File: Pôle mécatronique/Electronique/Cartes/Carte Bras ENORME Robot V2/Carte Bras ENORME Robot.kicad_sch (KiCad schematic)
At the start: 25 parts, among them Q1 BC557, U1 MCP2551-I-P, U2 IRFZ44NPBF

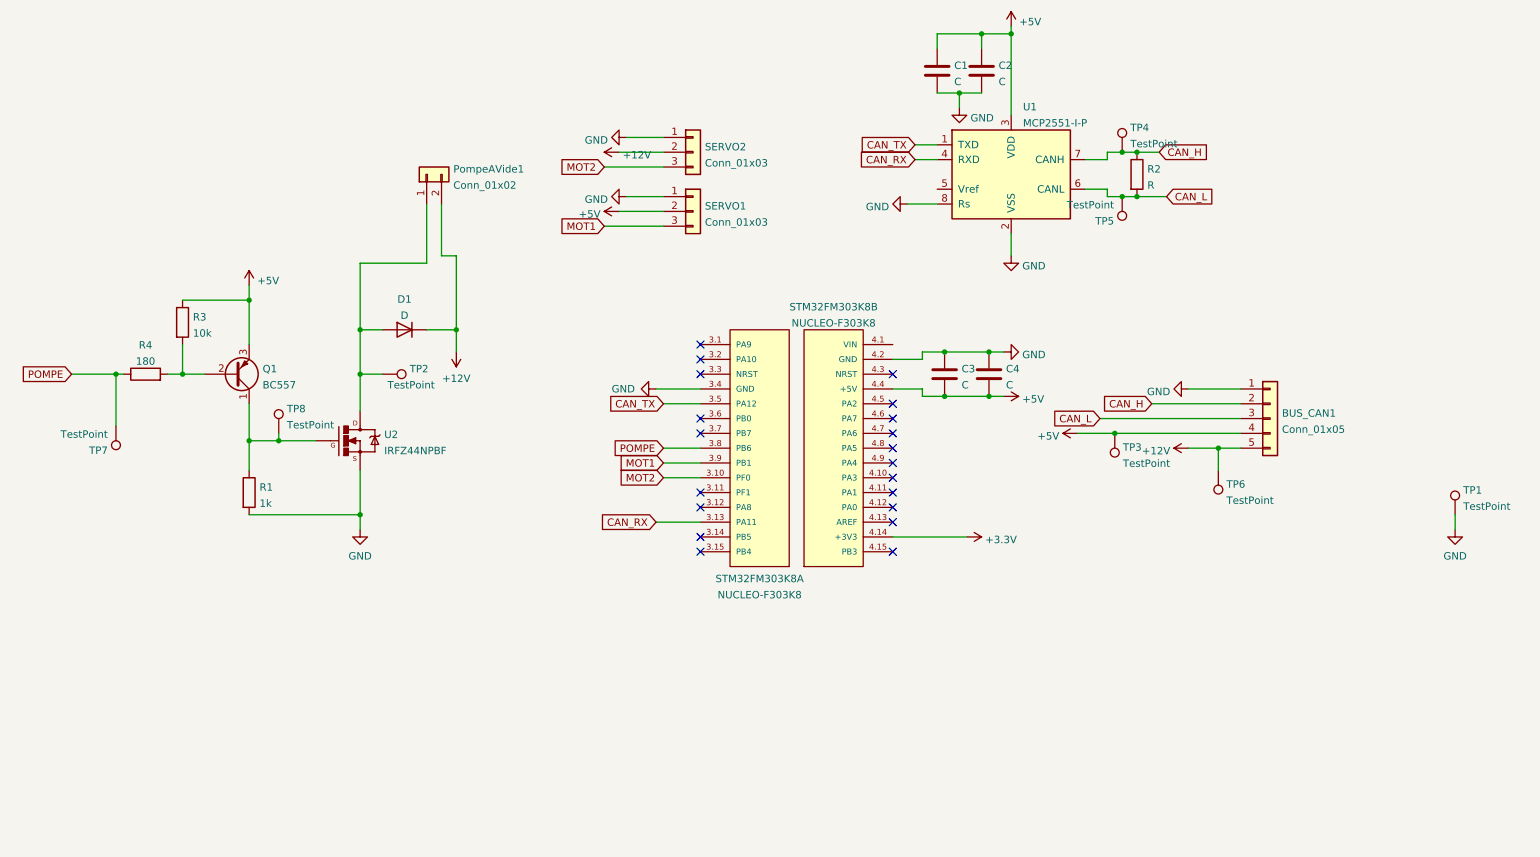
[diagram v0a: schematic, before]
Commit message: Up random
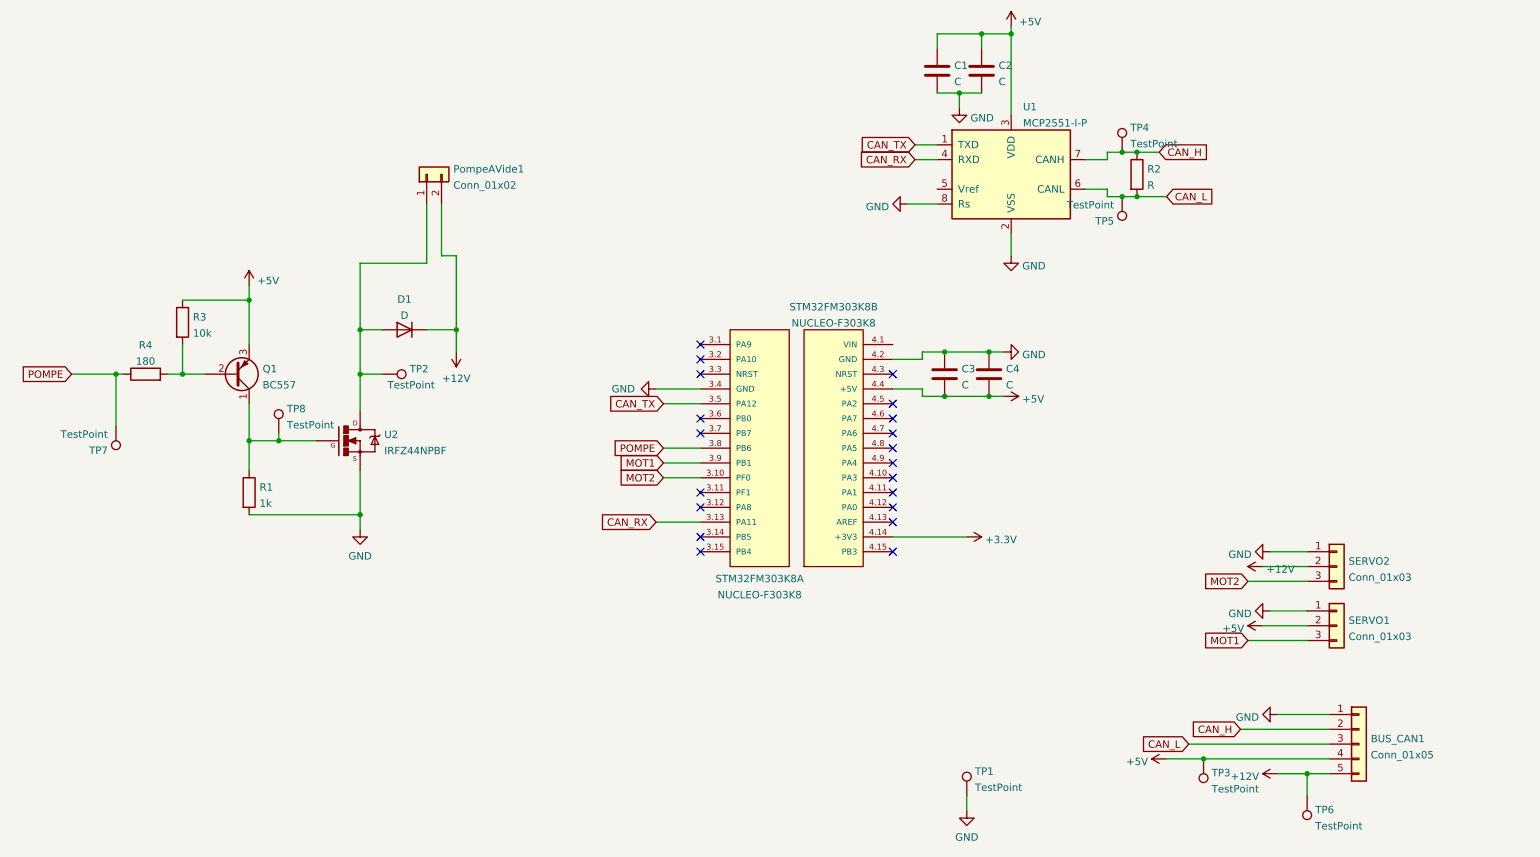
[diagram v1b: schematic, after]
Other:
- moved on the sheet: BUS_CAN1, SERVO1, SERVO2, TP1, TP3, TP6
